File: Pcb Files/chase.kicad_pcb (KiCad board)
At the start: 2 copper layers, 65.5 x 110 mm, 23 parts, among them P1 Conn_01x01_Pin, P2 Conn_01x01_Pin, P3 Conn_01x01_Pin, P4 Conn_01x01_Pin, P5 Conn_01x01_Pin, P6 Conn_01x01_Pin, P7 Conn_01x01_Pin, P8 Conn_01x01_Pin, P9 Conn_01x01_Pin, Q1 Q_NMOS, Q2 Q_NMOS, Q3 Q_NMOS, U1 ARDUINO_NANO

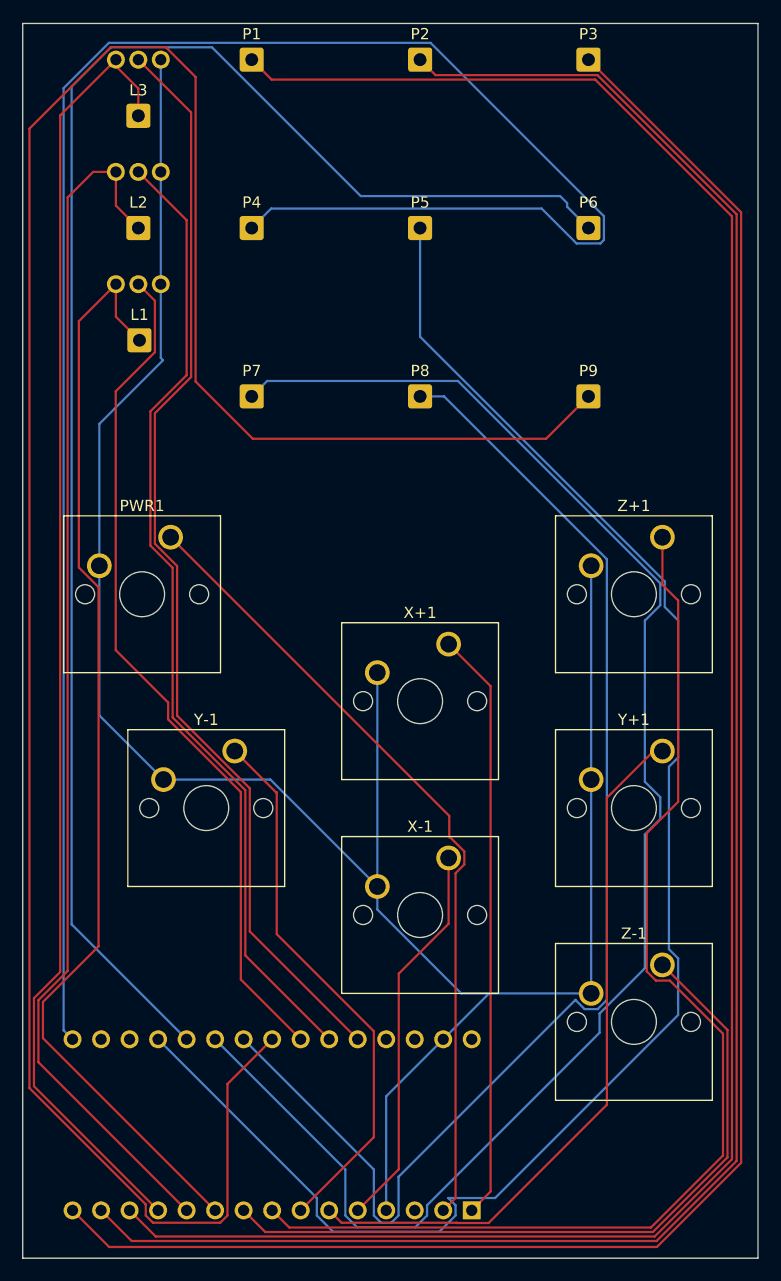
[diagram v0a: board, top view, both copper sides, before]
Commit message: Add files via upload
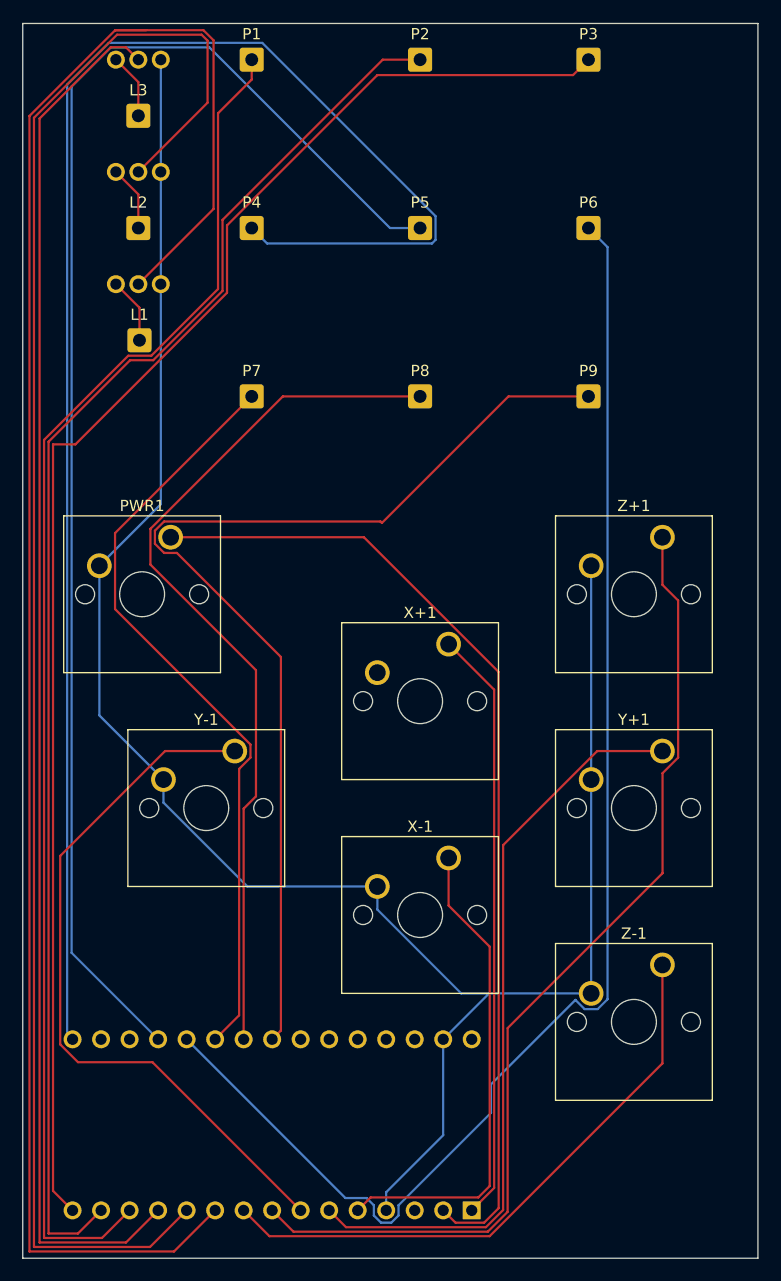
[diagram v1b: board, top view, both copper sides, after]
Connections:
- U1 pad 10: Net-(L1-Pin_1) -> /MOS1
- U1 pad 11: Net-(L2-Pin_1) -> /MOS2
- U1 pad 12: Net-(L3-Pin_1) -> /MOS3
- U1 pad 24: /MOS1 -> unconnected-(U1-A5-Pad24)
- U1 pad 25: /MOS2 -> unconnected-(U1-A6-Pad25)
- U1 pad 26: /MOS3 -> unconnected-(U1-A7-Pad26)
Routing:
- net Net-(P9-Pin_1): track 211.0 -> 94.6 mm
- net Net-(L3-Pin_1): track 115.9 -> 5.83 mm
- net Net-(L2-Pin_1): track 107.9 -> 5.83 mm
- net Net-(L1-Pin_1): track 98.9 -> 5.87 mm
- net /MOS1: track 76.2 -> 166.4 mm
- net Net-(P7-Pin_1): track 139.1 -> 68.6 mm
- net Net-(P1-Pin_1): track 190.0 -> 122.5 mm
- net /MOS2: track 87.0 -> 148.5 mm
- net Net-(P2-Pin_1): track 178.9 -> 127.0 mm
- net Net-(P8-Pin_1): track 114.4 -> 78.7 mm
- net Net-(P3-Pin_1): track 167.9 -> 134.4 mm
- net Net-(P4-Pin_1): track 176.9 -> 145.2 mm
- net /MOS3: track 98.0 -> 123.8 mm
- net Net-(P6-Pin_1): track 143.5 -> 125.2 mm
- net GND: track 196.4 -> 178.4 mm
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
